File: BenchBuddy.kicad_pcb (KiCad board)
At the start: 4 copper layers, 165.1 x 63.5 mm, 79 parts, among them K1 1461069-5, P1 24 Pin MiniFit JR, P2 CONN_3X2, P3 CONN_2, P4 12 Pin Terminal Block, P5 3 Pin TB, Q1 2N3904, Q2 DMN65D8L-7, Q3 AOD476, Q4 AOD476, SW1 Power Switch, U1 LTV-816S, U2 MCP3901, U3 LMT84, U4 OPA4170, U5 MCP4801

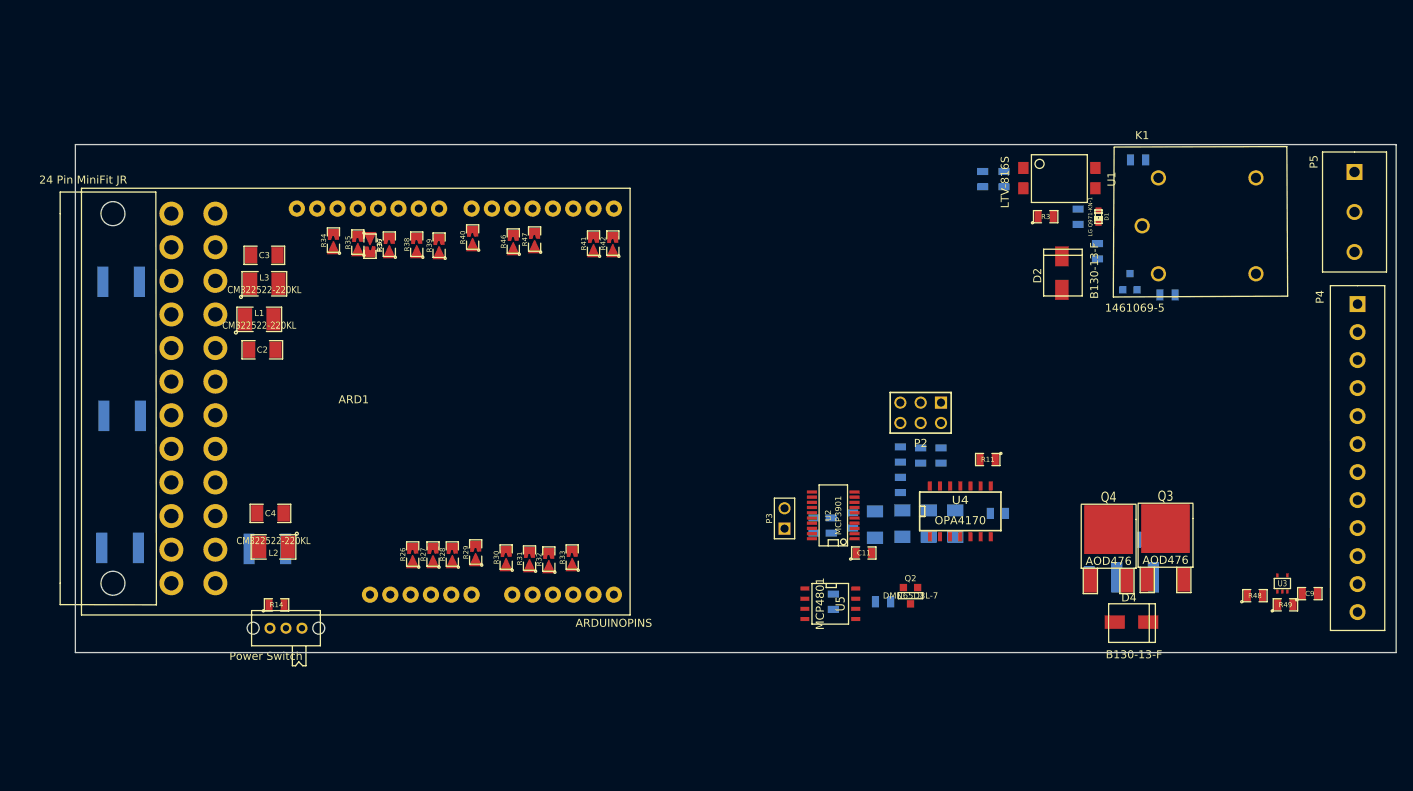
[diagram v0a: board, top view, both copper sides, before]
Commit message: Placing the Power Modify Module
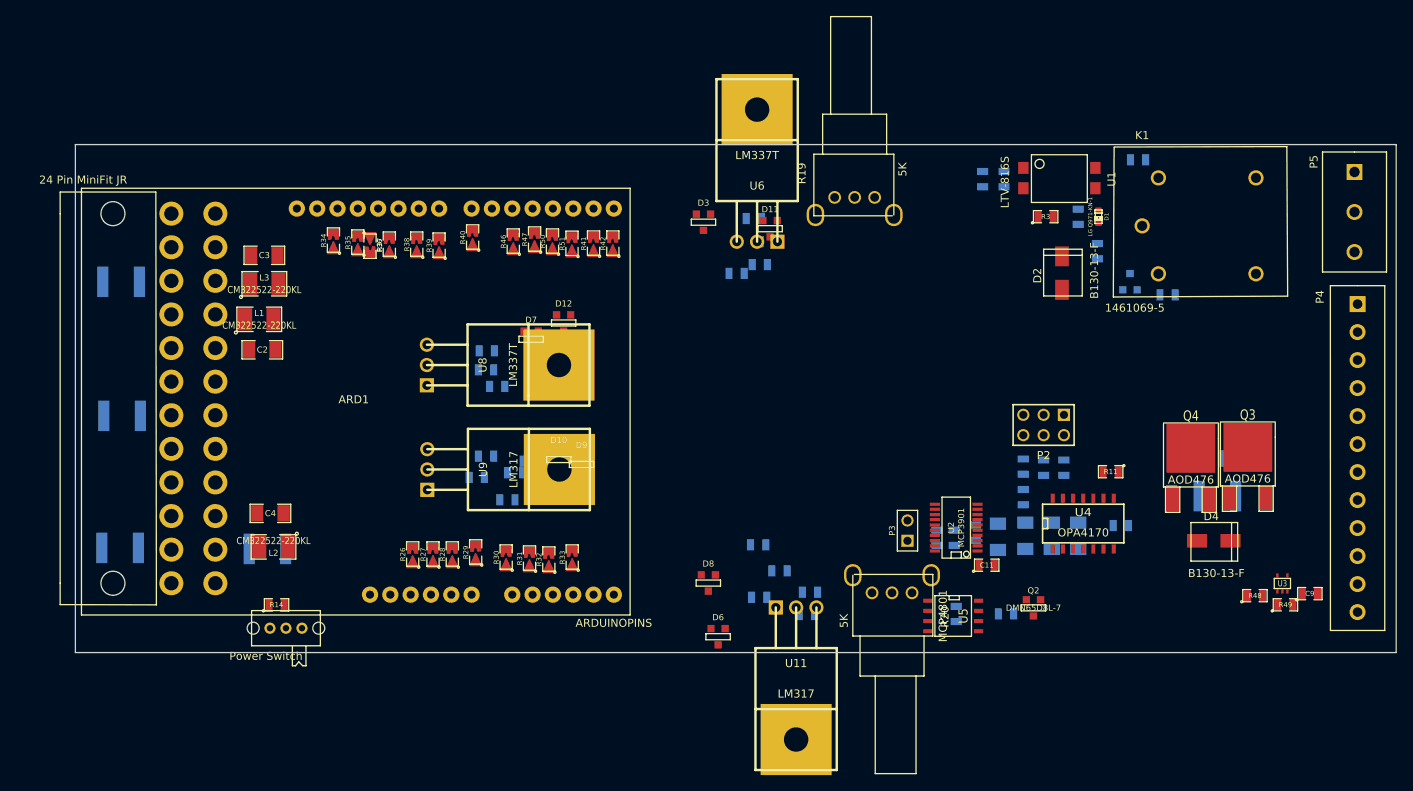
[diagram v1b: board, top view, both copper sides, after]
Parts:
- added C14: C, SM0805, B.Cu at (186.4, 137.4)
- added C15: C, SM0805, B.Cu at (187.6, 123.9)
- added C16: C, SM0805, B.Cu at (221.8, 110.8)
- added C17: C, SM0805, B.Cu at (224.3, 149.0)
- added C18: C, SM0805, B.Cu at (221.1, 105.0)
- added C19: C, SM0805, B.Cu at (228.1, 151.7)
- added C20: C, SM0805, B.Cu at (193.2, 135.3)
- added C21: C, SM0805, B.Cu at (193.7, 125.6)
- added C22: C, SM0805, B.Cu at (221.7, 152.3)
- added C23: C, SM0805, B.Cu at (199.3, 120.9)
- added C24: C, SM0805, B.Cu at (187.6, 134.7)
- added C25: C, SM0805, B.Cu at (199.6, 123.2)
- added D10: MMBD914-7-F, SOT23-DIODE, F.Cu at (196.7, 135.1)
- added D11: MMBD914-7-F, SOT23-DIODE, F.Cu at (223.1, 106.3)
- added D12: MMBD914-7-F, SOT23-DIODE, F.Cu at (197.3, 118.1)
- added D3: MMBD914-7-F, SOT23-DIODE, F.Cu at (214.8, 105.5)
- added D6: MMBD914-7-F, SOT23-DIODE, F.Cu at (216.6, 157.3)
- added D7: MMBD914-7-F, SOT23-DIODE, F.Cu at (193.2, 120.1)
- added D8: MMBD914-7-F, SOT23-DIODE, F.Cu at (215.4, 150.6)
- added D9: MMBD914-7-F, SOT23-DIODE, F.Cu at (199.5, 135.7)
- added R18: 715, SM0805, B.Cu at (222.8, 107.9)
- added R19: 5K, EVUE3K, F.Cu at (233.7, 102.4)
- added R20: 5K, EVUE3K, F.Cu at (238.4, 151.8)
- added R21: 715, SM0805, B.Cu at (227.7, 154.5)
- added R22: R, SM0805, B.Cu at (221.6, 145.8)
- added R23: R, SM0805, B.Cu at (195.2, 133.1)
- added R24: R, SM0805, B.Cu at (199.5, 125.7)
- added R25: R, SM0805, B.Cu at (218.9, 111.9)
- added R50: R, SM0805-blob, F.Cu at (195.9, 107.8)
- added R51: R, SM0805-blob, F.Cu at (198.3, 108.1)
- added R52: R, SM0805, B.Cu at (189.0, 126.0)
- added R53: R, SM0805, B.Cu at (187.7, 121.5)
- added R54: R, SM0805, B.Cu at (191.2, 136.8)
- added R55: R, SM0805, B.Cu at (190.3, 140.2)
- added U11: LM317, TO220, F.Cu at (226.4, 153.6)
- added U6: LM337T, TO220, F.Cu at (221.5, 107.9)
- added U8: LM337T, TO220, F.Cu at (180.2, 123.3)
- added U9: LM317, TO220, F.Cu at (180.3, 136.4)
- moved C1 15.4 mm to (248.8, 144.3)
- moved C10 15.4 mm to (267.0, 143.4)
- moved C7 15.4 mm to (244.0, 144.9)
- moved C8 15.4 mm to (246.1, 144.9)
- moved P2 15.4 mm to (257.3, 130.8)
- moved R10 15.4 mm to (261.6, 144.7)
- moved R11 15.4 mm to (265.7, 136.7)
- moved R15 15.4 mm to (252.6, 154.4)
- moved R45 15.4 mm to (257.3, 136.1)
- moved C11 15.4 mm to (250.2, 148.3)
- moved C12 15.4 mm to (246.4, 154.4)
- moved P3 15.4 mm to (240.3, 144.0)
- moved Q2 15.4 mm to (256.0, 153.7)
- moved R12 15.4 mm to (259.8, 136.1)
- moved R13 15.4 mm to (254.8, 139.8)
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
